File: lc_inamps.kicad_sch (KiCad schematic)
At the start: 30 parts, among them J14 Conn_01x04_Female, J15 Conn_01x04_Female, J16 Conn_01x08_Female, J17 Conn_01x04_Female, J18 Conn_01x04_Female, J6 Conn_01x04_Female, U3 MCP6N11T-001E, U4 MCP6N11T-001E, U5 MCP6N11T-001E, U6 MCP6N11T-001E

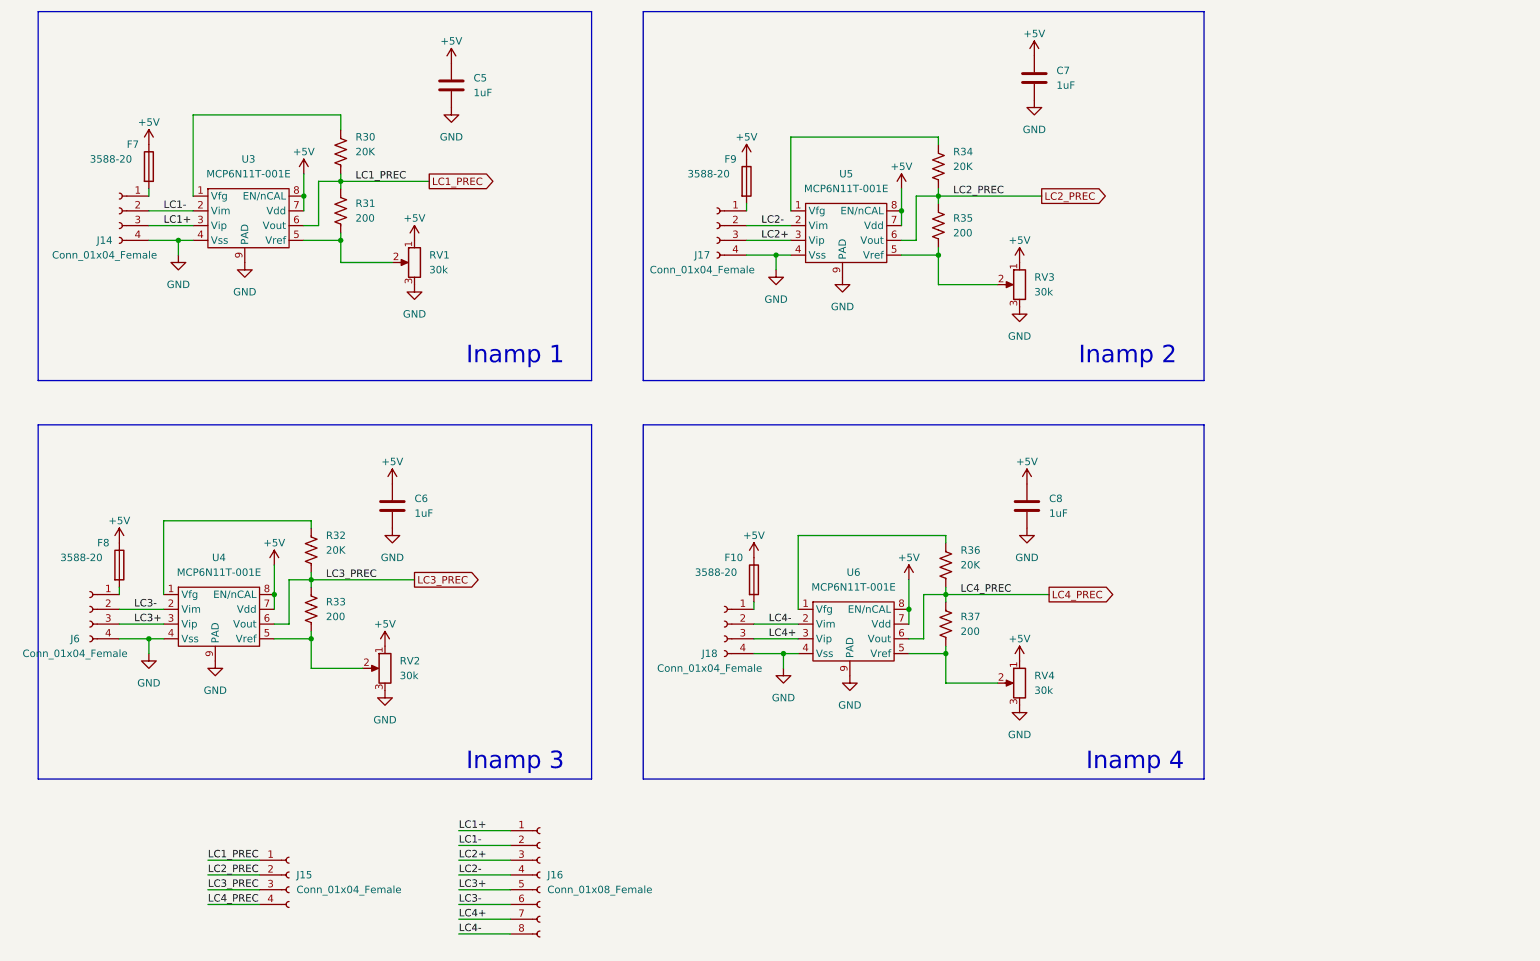
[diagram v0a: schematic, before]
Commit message: preliminary layout and started pwr plane config
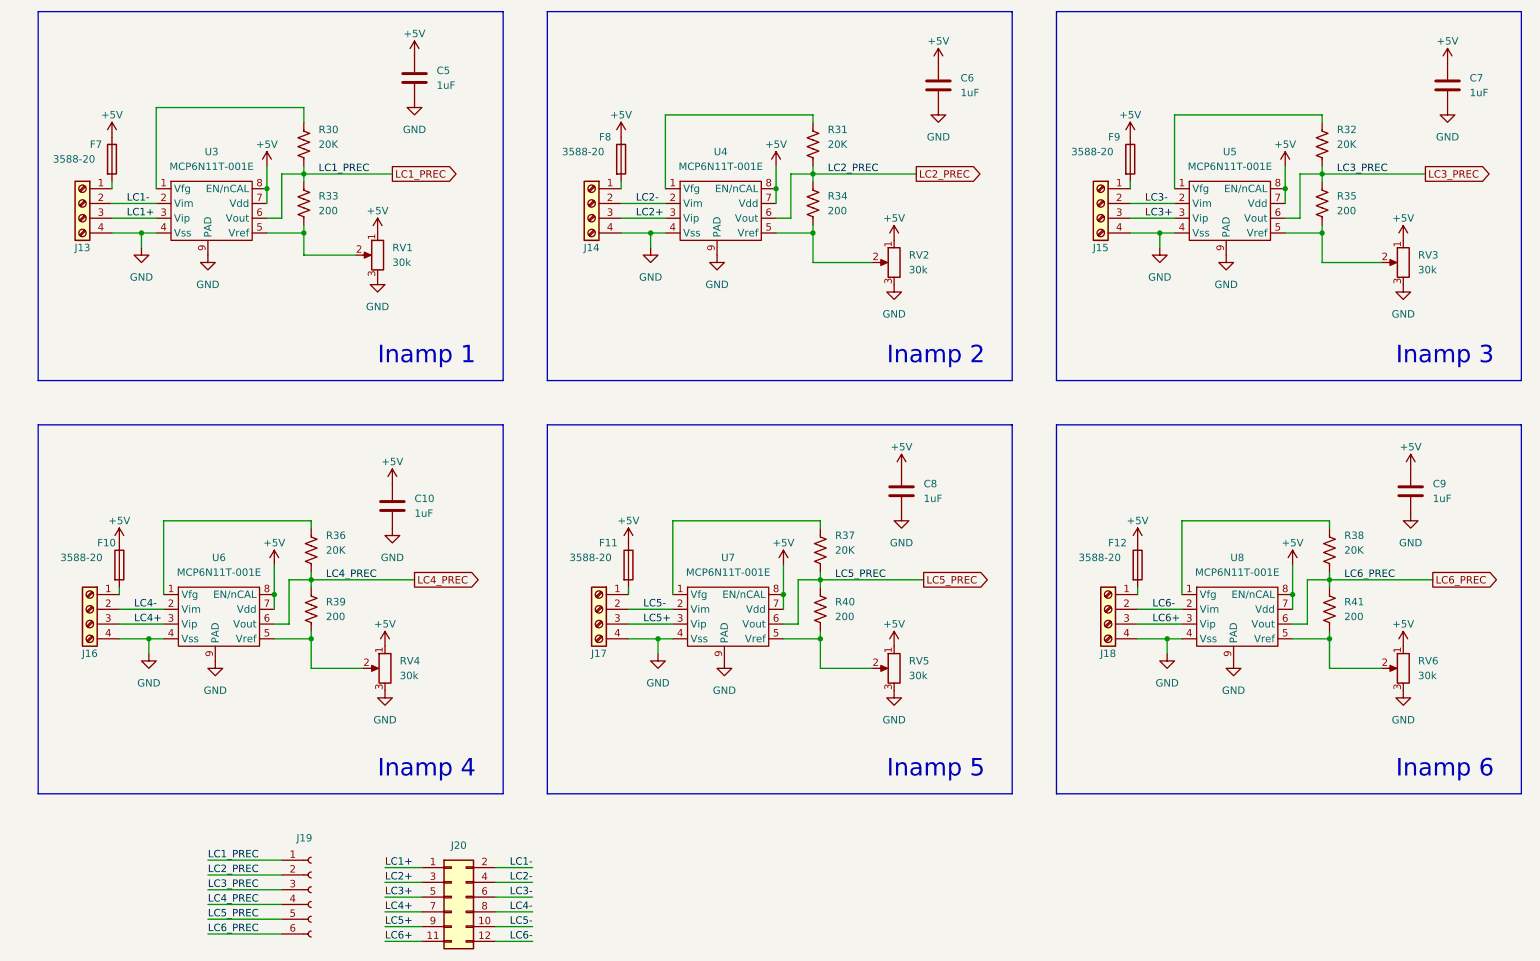
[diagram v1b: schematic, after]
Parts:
- removed J14, J17, J18, J6: Conn_01x04_Female, karca_custom_footprints:LPTA-4pos, symbol Connector:Conn_01x04_Female
- removed J15: Conn_01x04_Female, Connector_PinHeader_2.54mm:PinHeader_1x04_P2.54mm_Vertical, symbol Connector:Conn_01x04_Female
- removed J16: Conn_01x08_Female, Connector_PinSocket_2.54mm:PinSocket_1x08_P2.54mm_Vertical, symbol Connector:Conn_01x08_Female
- added C7, C9: 1uF, Capacitor_SMD:C_1206_3216Metric, symbol Device:C
- added F12, F9: 3588-20, 3588-20:358820, symbol Device:Fuse
- added J13, J14, J15, J16, J17, J18: Screw_Terminal_01x04, 1190365:1190365, symbol Connector:Screw_Terminal_01x04
- added J19: Conn_01x06_Female, Connector_PinSocket_2.54mm:PinSocket_1x06_P2.54mm_Vertical, symbol Connector:Conn_01x06_Female
- added J20: Conn_02x06_Odd_Even, Connector_PinSocket_2.54mm:PinSocket_2x06_P2.54mm_Vertical, symbol Connector_Generic:Conn_02x06_Odd_Even
- added R32, R38: 20K, Resistor_SMD:R_1206_3216Metric, symbol Device:R_US
- added R35, R41: 200, Resistor_SMD:R_1206_3216Metric, symbol Device:R_US
- added RV3, RV6: 30k, 3296W-1-303LF:TRIM_3296W-1-303LF, symbol Device:R_Potentiometer
- added U5, U8: MCP6N11T-001E, Package_DFN_QFN:TDFN-8-1EP_3x2mm_P0.5mm_EP1.80x1.65mm, symbol karca_custom_components:MCP6N11R
- F10: renamed from F8; footprint karca_custom_footprints:3588-20 fuse -> 3588-20:358820
- F11: renamed from F10; footprint karca_custom_footprints:3588-20 fuse -> 3588-20:358820
- F7: footprint karca_custom_footprints:3588-20 fuse -> 3588-20:358820
- F8: renamed from F9; footprint karca_custom_footprints:3588-20 fuse -> 3588-20:358820
- renumbered C6 to C10, C7 to C6, R34 to R31, R31 to R33, R35 to R34, R32 to R36, R36 to R37, R33 to R39, R37 to R40, RV3 to RV2, RV2 to RV4, RV4 to RV5, U5 to U4, U4 to U6, U6 to U7
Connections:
- net +5V: now also C7.1, C9.1, F12.1, F9.1, RV3.1, RV6.1, U5.7 (Vdd), U5.8 (EN/nCAL), U8.7 (Vdd), U8.8 (EN/nCAL)
- net GND: now also C7.2, C9.2, J13.4 (Pin_4), J14.4 (Pin_4), J15.4 (Pin_4), J16.4 (Pin_4), J17.4 (Pin_4), J18.4 (Pin_4), RV3.3, RV6.3, U5.4 (Vss), U5.9 (PAD), U8.4 (Vss), U8.9 (PAD)
- net LC1+: now also J13.3 (Pin_3), J20.1 (Pin_1)
- net LC1-: now also J13.2 (Pin_2), J20.2 (Pin_2)
- net LC1_PREC: now also J19.1 (Pin_1)
- net LC2+: now also J14.3 (Pin_3), J20.3 (Pin_3)
- net LC2-: now also J14.2 (Pin_2), J20.4 (Pin_4)
- net LC2_PREC: now also J19.2 (Pin_2)
- net LC3+: now also J15.3 (Pin_3), J20.5 (Pin_5), U5.3 (Vip); no longer U6.3 (Vip)
- net LC3-: now also J15.2 (Pin_2), J20.6 (Pin_6), U5.2 (Vim); no longer U6.2 (Vim)
- net LC3_PREC: now also J19.3 (Pin_3), R32.1, R35.2, U5.6 (Vout); no longer R36.1, R39.2, U6.6 (Vout)
- net LC4+: now also U6.3 (Vip), J16.3 (Pin_3), J20.7 (Pin_7); no longer U7.3 (Vip)
- net LC4-: now also U6.2 (Vim), J16.2 (Pin_2), J20.8 (Pin_8); no longer U7.2 (Vim)
- net LC4_PREC: now also R36.1, R39.2, U6.6 (Vout), J19.4 (Pin_4); no longer R37.1, R40.2, U7.6 (Vout)
- net at F7.2: now also J13.1 (Pin_1)
- net at F11.2: now also J17.1 (Pin_1)
- net at F10.2: now also J16.1 (Pin_1)
- net at F8.2: now also J14.1 (Pin_1)
- new net: R32.2, U5.1 (Vfg)
- new net: R35.1, RV3.2, U5.5 (Vref)
- new net: F12.2, J18.1 (Pin_1)
- new net: R38.2, U8.1 (Vfg)
- new net: R41.1, RV6.2, U8.5 (Vref)
- new net: F9.2, J15.1 (Pin_1)
- new net LC5+: J17.3 (Pin_3), J20.9 (Pin_9), U7.3 (Vip)
- new net LC5-: J17.2 (Pin_2), J20.10 (Pin_10), U7.2 (Vim)
- new net LC5_PREC: J19.5 (Pin_5), R37.1, R40.2, U7.6 (Vout)
- new net LC6+: J18.3 (Pin_3), J20.11 (Pin_11), U8.3 (Vip)
- new net LC6-: J18.2 (Pin_2), J20.12 (Pin_12), U8.2 (Vim)
- new net LC6_PREC: J19.6 (Pin_6), R38.1, R41.2, U8.6 (Vout)
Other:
- note added: "Inamp 5"
- note added: "Inamp 6"
- moved on the sheet: C5, C6, C8, F11, F7, F8, R30, R31, R33, R34, R37, R40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
